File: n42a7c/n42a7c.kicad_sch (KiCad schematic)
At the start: 112 parts, among them J1 S2B-PH-SM4-TB, SW1 CPG151101S11-16, SW10 CPG151101S11-16, SW11 CPG151101S11-16, SW12 CPG151101S11-16, SW13 CPG151101S11-16, SW14 CPG151101S11-16, SW15 CPG151101S11-16, SW16 CPG151101S11-16, SW17 CPG151101S11-16, SW18 CPG151101S11-16, SW19 CPG151101S11-16, SW2 CPG151101S11-16, SW20 CPG151101S11-16, SW21 CPG151101S11-16, SW22 CPG151101S11-16, SW23 CPG151101S11-16, SW24 CPG151101S11-16, SW25 CPG151101S11-16, SW26 CPG151101S11-16, SW27 CPG151101S11-16, SW28 CPG151101S11-16, SW29 CPG151101S11-16, SW3 CPG151101S11-16, SW30 CPG151101S11-16, SW31 CPG151101S11-16, SW32 CPG151101S11-16, SW33 CPG151101S11-16, SW34 CPG151101S11-16, SW35 CPG151101S11-16, SW36 CPG151101S11-16, SW37 CPG151101S11-16, SW38 CPG151101S11-16, SW39 CPG151101S11-16, SW4 CPG151101S11-16, SW40 CPG151101S11-16, SW41 CPG151101S11-16, SW42 CPG151101S11-16, SW5 CPG151101S11-16, SW6 CPG151101S11-16, SW7 CPG151101S11-16, SW8 CPG151101S11-16, SW9 CPG151101S11-16, U1 XIAO-nRF52840-SMD

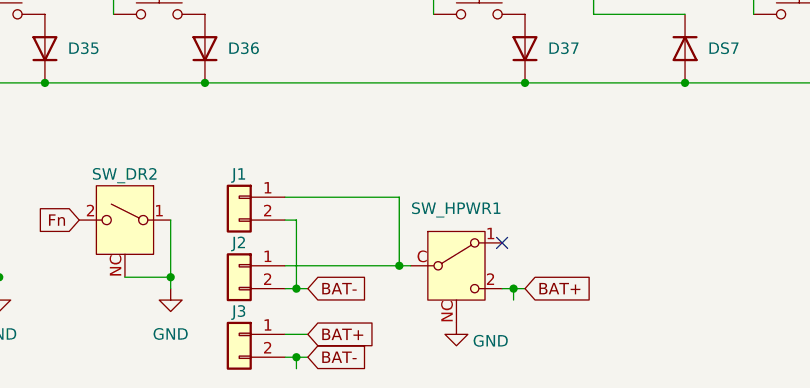
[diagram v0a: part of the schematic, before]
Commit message: revise switch
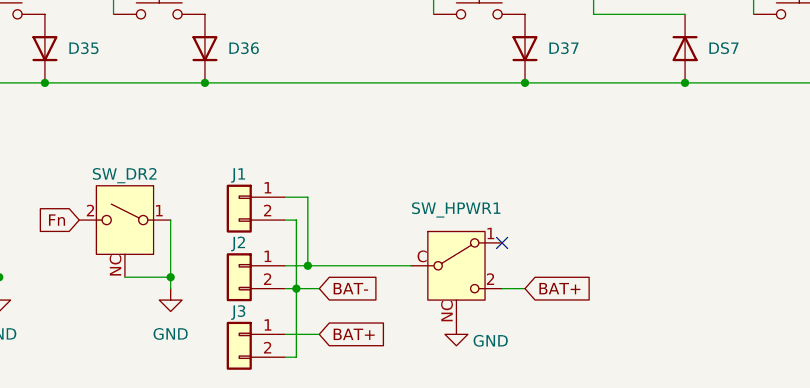
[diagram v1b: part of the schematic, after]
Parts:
- J2, J3: value (none) -> ~
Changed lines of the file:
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@@
 	)
 	(junction
-		(at 86.36 179.07)
-		(diameter 0)
-		(color 0 0 0 0)
-	)
-	(junction
 		(at 29.21 177.8)
 		(diameter 0)
@@
 	)
 	(junction
-		(at 62.23 186.69)
-		(diameter 0)
-		(color 0 0 0 0)
-	)
-	(junction
 		(at 219.71 130.81)
 		(diameter 0)
@@
 	)
 	(junction
+		(at 63.5 176.53)
+		(diameter 0)
+		(color 0 0 0 0)
+	)
+	(junction
 		(at 184.15 113.03)
 		(diameter 0)
@@
 	)
 	(junction
-		(at 73.66 176.53)
-		(diameter 0)
-		(color 0 0 0 0)
-	)
-	(junction
 		(at 229.87 138.43)
 		(diameter 0)
@@
 	(wire
 		(pts
-			(xy 60.96 176.53) (xy 73.66 176.53)
+			(xy 60.96 176.53) (xy 63.5 176.53)
 		)
 		(stroke
@@
 	(wire
 		(pts
-			(xy 62.23 186.69) (xy 62.23 187.96)
+			(xy 63.5 168.91) (xy 63.5 176.53)
 		)
 		(stroke
@@
 	(wire
 		(pts
-			(xy 73.66 176.53) (xy 73.66 168.91)
-		)
-		(stroke
-			(width 0)
-			(type default)
-		)
-	)
-	(wire
-		(pts
 			(xy 69.85 102.87) (xy 52.07 102.87)
 		)
@@
 	(wire
 		(pts
-			(xy 86.36 179.07) (xy 86.36 180.34)
-		)
-		(stroke
-			(width 0)
-			(type default)
-		)
-	)
-	(wire
-		(pts
 			(xy 95.25 130.81) (xy 95.25 148.59)
 		)
@@
 	(wire
 		(pts
-			(xy 73.66 176.53) (xy 74.93 176.53)
+			(xy 63.5 168.91) (xy 60.96 168.91)
 		)
 		(stroke
@@
 	(wire
 		(pts
-			(xy 73.66 168.91) (xy 60.96 168.91)
+			(xy 229.87 120.65) (xy 255.27 120.65)
 		)
 		(stroke
@@
 	(wire
 		(pts
-			(xy 229.87 120.65) (xy 255.27 120.65)
+			(xy 139.7 85.09) (xy 139.7 95.25)
 		)
 		(stroke
@@
 	(wire
 		(pts
-			(xy 139.7 85.09) (xy 139.7 95.25)
+			(xy 275.59 148.59) (xy 273.05 148.59)
 		)
 		(stroke
@@
 	(wire
 		(pts
-			(xy 275.59 148.59) (xy 273.05 148.59)
+			(xy 275.59 95.25) (xy 273.05 95.25)
 		)
 		(stroke
@@
 	(wire
 		(pts
-			(xy 275.59 95.25) (xy 273.05 95.25)
+			(xy 194.31 138.43) (xy 212.09 138.43)
 		)
 		(stroke
@@
 	(wire
 		(pts
-			(xy 194.31 138.43) (xy 212.09 138.43)
+			(xy 63.5 176.53) (xy 74.93 176.53)
 		)
 		(stroke
@@
 	(wire
 		(pts
-			(xy 86.36 179.07) (xy 87.63 179.07)
+			(xy 85.09 179.07) (xy 87.63 179.07)
 		)
 		(stroke
@@
 	(wire
 		(pts
-			(xy 62.23 186.69) (xy 63.5 186.69)
+			(xy 62.23 179.07) (xy 64.77 179.07)
 		)
 		(stroke
@@
 	(wire
 		(pts
-			(xy 62.23 179.07) (xy 63.5 179.07)
-		)
-		(stroke
-			(width 0)
-			(type default)
-		)
-	)
-	(wire
-		(pts
 			(xy 87.63 138.43) (xy 69.85 138.43)
 		)
@@
 	(wire
 		(pts
-			(xy 85.09 179.07) (xy 86.36 179.07)
-		)
-		(stroke
-			(width 0)
-			(type default)
-		)
-	)
-	(wire
-		(pts
 			(xy 69.85 138.43) (xy 52.07 138.43)
 		)
@@
 	(wire
 		(pts
-			(xy 60.96 184.15) (xy 63.5 184.15)
+			(xy 60.96 184.15) (xy 64.77 184.15)
 		)
 		(stroke
@@
 		)
 	)
+	(wire
+		(pts
+			(xy 62.23 179.07) (xy 62.23 186.69)
+		)
+		(stroke
+			(width 0)
+			(type default)
+		)
+	)
 	(global_label "IO 0"
 		(shape bidirectional)
@@
 	(global_label "BAT-"
 		(shape input)
-		(at 63.5 186.69 0)
+		(at 64.77 179.07 0)
 		(effects
 			(font
@@
 		)
 		(property "Intersheetrefs" "${INTERSHEET_REFS}"
-			(at 63.5 186.69 90)
+			(at 64.77 179.07 90)
 			(effects
 				(font
@@
 		)
 	)
-	(global_label "BAT-"
-		(shape input)
-		(at 63.5 179.07 0)
-		(fields_autoplaced yes)
-		(effects
-			(font
-				(size 1.27 1.27)
-			)
-			(justify left)
-		)
-		(property "Intersheetrefs" "${INTERSHEET_REFS}"
-			(at 70.7296 179.07 0)
-			(effects
-				(font
-					(size 1.27 1.27)
-				)
-				(justify left)
-				(hide yes)
-			)
-		)
-	)
 	(global_label "IO 2"
 		(shape bidirectional)
@@
 	(global_label "BAT+"
 		(shape input)
-		(at 63.5 184.15 0)
+		(at 64.77 184.15 0)
 		(effects
 			(font
@@
 		)
 		(property "Intersheetrefs" "${INTERSHEET_REFS}"
-			(at 63.5 184.15 90)
+			(at 64.77 184.15 90)
 			(effects
 				(font
@@
 		)
 	)
-	(netclass_flag ""
-		(length 2.54)
-		(shape round)
-		(at 86.36 180.34 180)
-		(fields_autoplaced yes)
-		(effects
-			(font
-				(size 1.27 1.27)
-			)
-			(justify right bottom)
-		)
-		(property "Netclass" "Power"
-			(at 86.9696 182.88 0)
-			(effects
-				(font
-					(size 1.27 1.27)
-				)
-				(justify left)
-			)
-		)
-		(property "Component Class" ""
-			(at 182.88 22.86 0)
-			(effects
-				(font
-					(size 1.27 1.27)
-					(italic yes)
-				)
-				(justify left)
-			)
-		)
-	)
-	(netclass_flag ""
-		(length 2.54)
-		(shape round)
-		(at 73.66 176.53 180)
-		(fields_autoplaced yes)
-		(effects
-			(font
-				(size 1.27 1.27)
-			)
-			(justify right bottom)
-		)
-		(property "Netclass" "Power"
-			(at 74.2696 179.07 0)
-			(effects
-				(font
-					(size 1.27 1.27)
-				)
-				(justify left)
-			)
-		)
-		(property "Component Class" ""
-			(at 170.18 19.05 0)
-			(effects
-				(font
-					(size 1.27 1.27)
-					(italic yes)
-				)
-				(justify left)
-			)
-		)
-	)
-	(netclass_flag ""
-		(length 2.54)
-		(shape round)
-		(at 62.23 187.96 180)
-		(fields_autoplaced yes)
-		(effects
-			(font
-				(size 1.27 1.27)
-			)
-			(justify right bottom)
-		)
-		(property "Netclass" "Power"
-			(at 62.8396 190.5 0)
-			(effects
-				(font
-					(size 1.27 1.27)
-				)
-				(justify left)
-			)
-		)
-		(property "Component Class" ""
-			(at 158.75 30.48 0)
-			(effects
-				(font
-					(size 1.27 1.27)
-					(italic yes)
-				)
-				(justify left)
-			)
-		)
-	)
 	(symbol
 		(lib_id "power:PWR_FLAG")
@@
 			)
 		)
-		(property "Value" ""
+		(property "Value" "~"
 			(at 55.88 182.88 0)
 			(effects
@@
 			)
 		)
-		(property "Value" ""
+		(property "Value" "~"
 			(at 55.88 190.5 0)
 			(effects
